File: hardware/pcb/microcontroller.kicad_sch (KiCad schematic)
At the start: 44 parts, among them J3 TYPE-C sinking plate, Q1 2N7002VC-, Q2 2N7002VC-, SW18 SWITCH, U1 W25Q64JV, U3 USBLC6-2P6, U4 XC6206P332MR-G, U6 RP2040, U7 74LVC1T45, Y1 12MHz

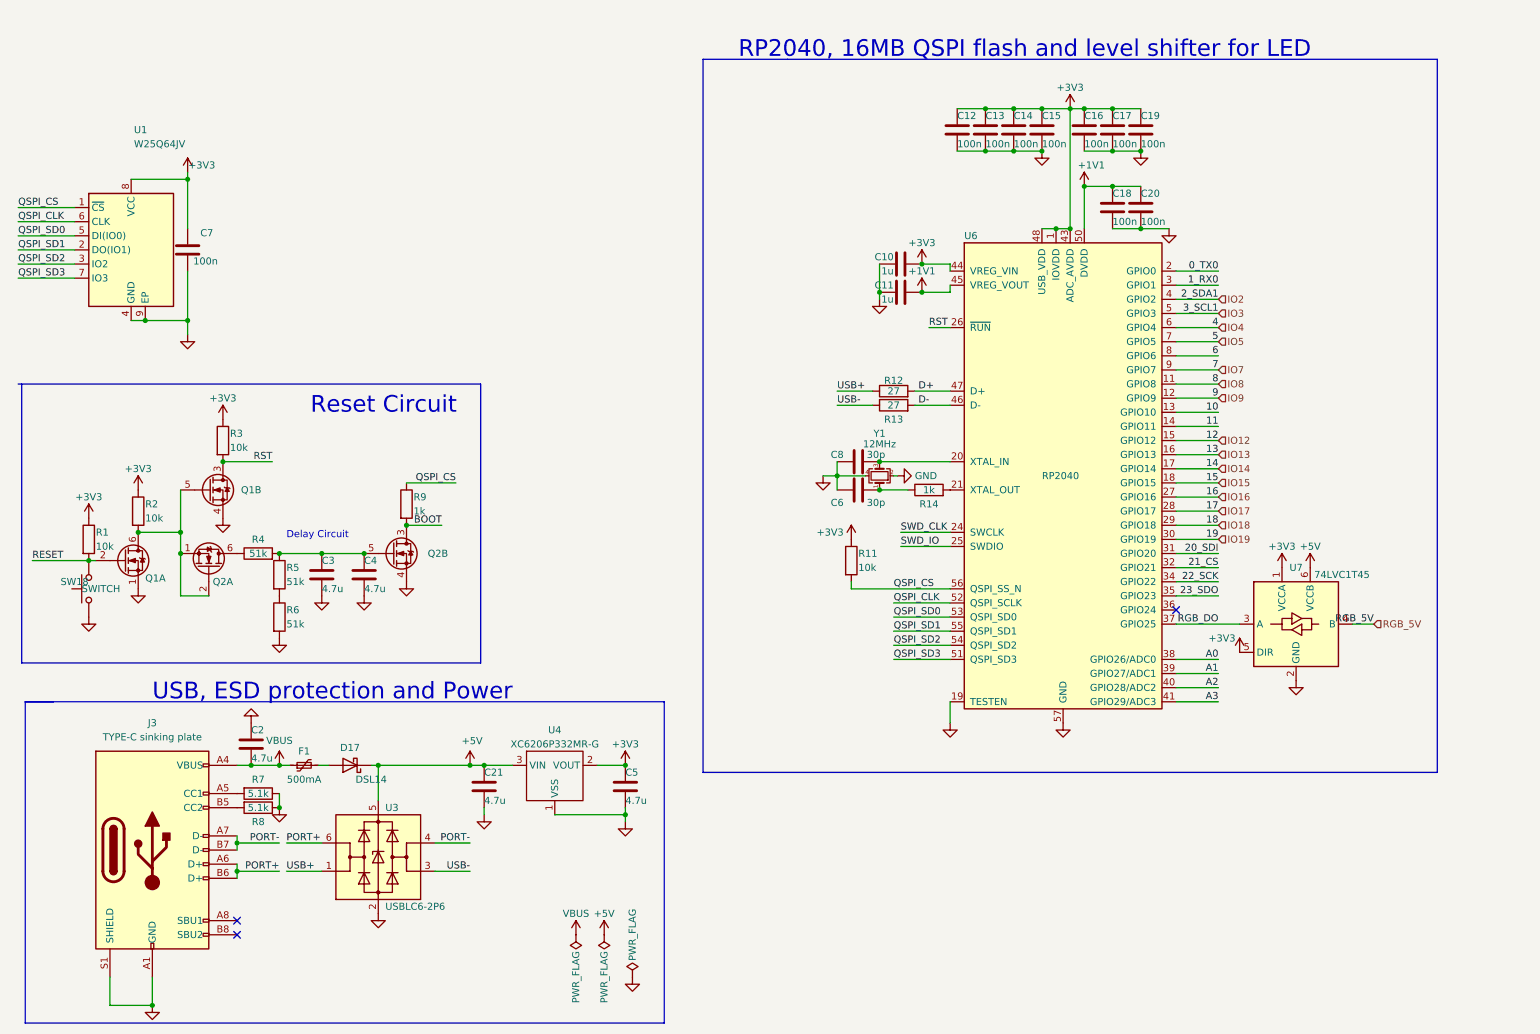
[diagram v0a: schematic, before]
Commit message: V1.5
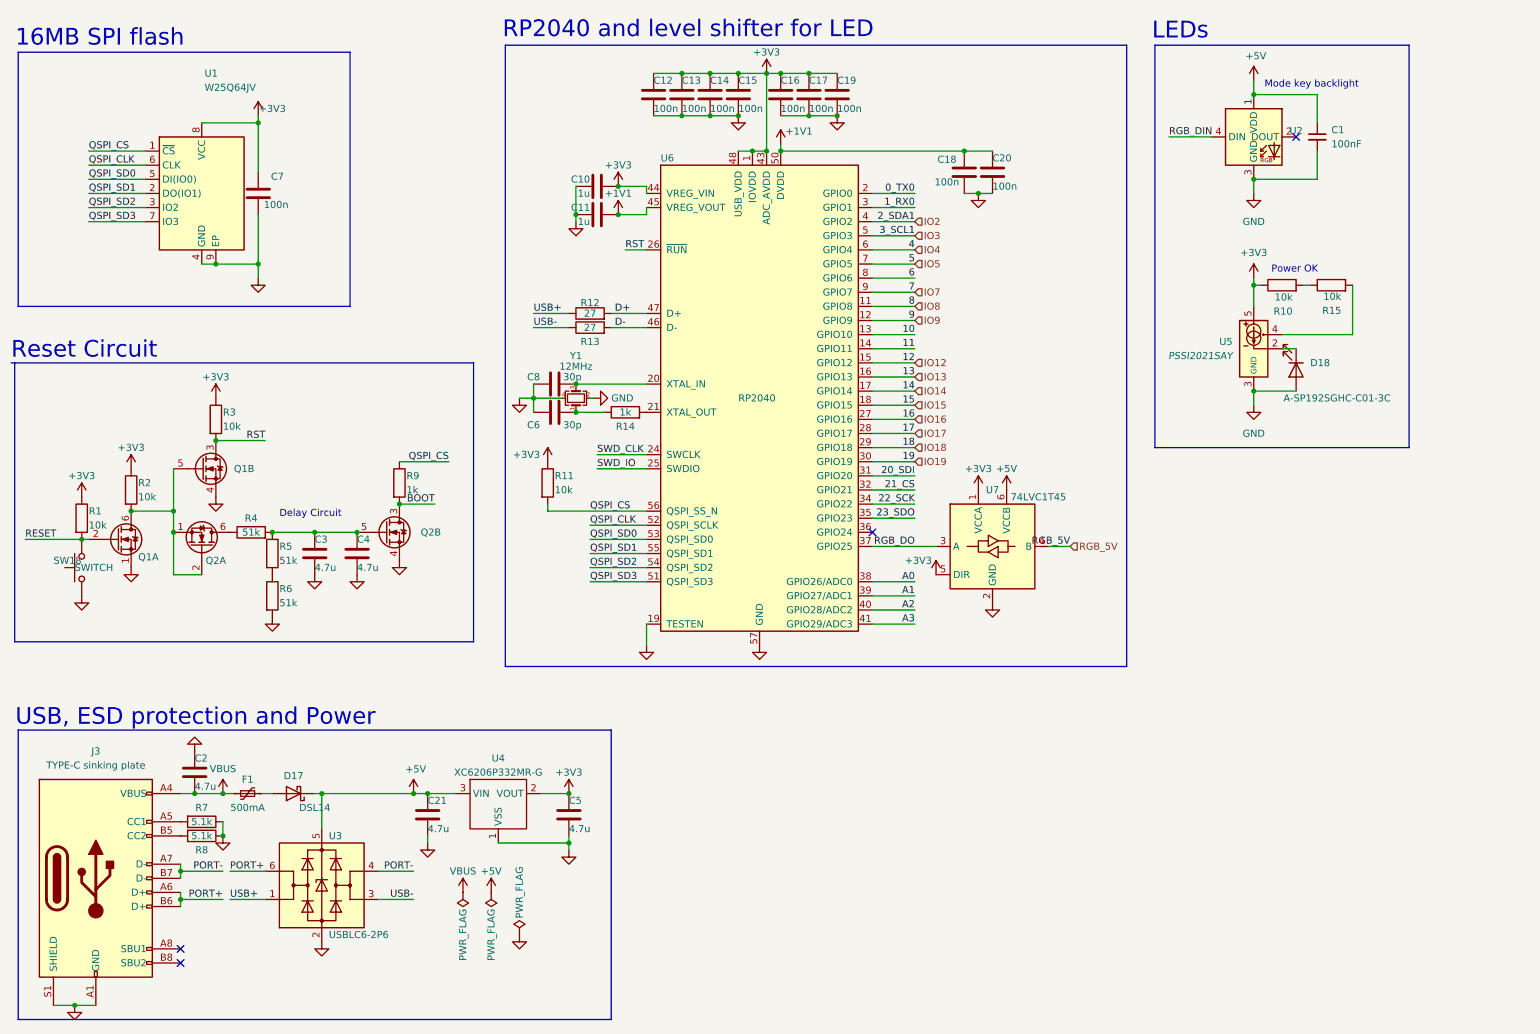
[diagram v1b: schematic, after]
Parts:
- added C1: 100nF, Capacitor_SMD:C_0603_1608Metric, symbol Device:C_Small
- added D18: A-SP192SGHC-C01-3C, mathboard:LED_SMD_0603_flat, symbol Device:LED
- added R10, R15: 10k, Resistor_SMD:R_0402_1005Metric, symbol Device:R
- added U2: ~, mathboard:SK6812-MINI-E, symbol Mathboard:SK6812MINI-E
- added U5: PSSI2021SAY, Package_TO_SOT_SMD:SOT-353_SC-70-5, symbol Reference_Current:PSSI2021SAY
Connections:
- net +3V3: now also R10.1, U5.5
- net +5V: now also C1.1, U2.1 (VDD)
- net GND: now also C1.2, D18.2 (A), U2.3 (GND), U5.3 (GND)
- new net: R10.2, R15.1
- new net: R15.2, U5.4
- new net: D18.1 (K), U5.2
- new net RGB_DIN: U2.4 (DIN)
- no-connect marks 3 -> 4
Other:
- note added: "16MB SPI flash"
- note added: "LEDs"
- note added: "Mode key backlight"
- note added: "Power OK"
- note added: "RP2040 and level shifter for LED"
- note removed: "RP2040, 16MB QSPI flash and level shifter for LED"
- title: (none) -> Mathboard 
- moved on the sheet: C10, C11, C12, C13, C14, C15, C16, C17, C18, C19, C2, C20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
